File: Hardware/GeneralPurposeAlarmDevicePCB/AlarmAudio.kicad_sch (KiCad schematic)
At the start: 18 parts, among them J601 22-23-2021, J602 22-23-2021, Q601 BSS138, Q602 DNI

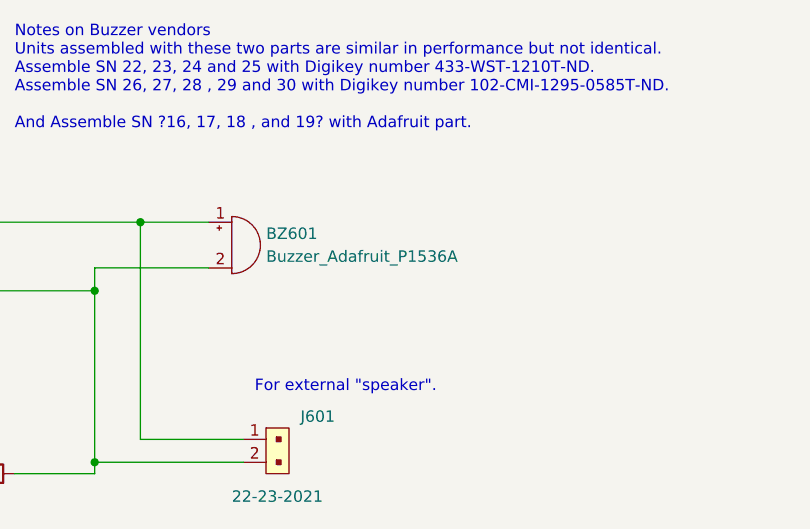
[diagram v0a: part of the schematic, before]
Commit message: Update the part number for the buzzer to a DigiKey part. This schematic is now saved in KiCAD 7.
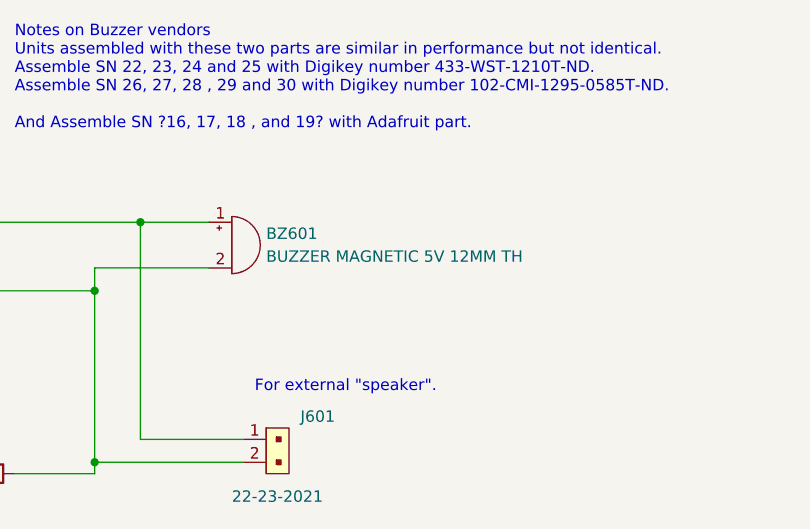
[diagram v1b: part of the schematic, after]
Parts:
- BZ601: value Buzzer_Adafruit_P1536A -> BUZZER MAGNETIC 5V 12MM TH; Cost .98 -> 0.83000; Distributor 1 Adafruit -> Digikey; Distributor 1 PN P1536A -> 433-WST-1210T-ND; MPN PS1240P02BT -> WST-1210T; Manufacturer (none) -> Soberton Inc.
